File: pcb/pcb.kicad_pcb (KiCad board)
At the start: 2 copper layers, 32 x 39 mm, 88 parts, among them U1 JM20330, U2 SM2258XT, U3 FlashBGA152, U4 Conn_41PIN, U5 SY8008, U6 SY8008, U7 TX4314, Y1 25MHz, Y2 50MHz

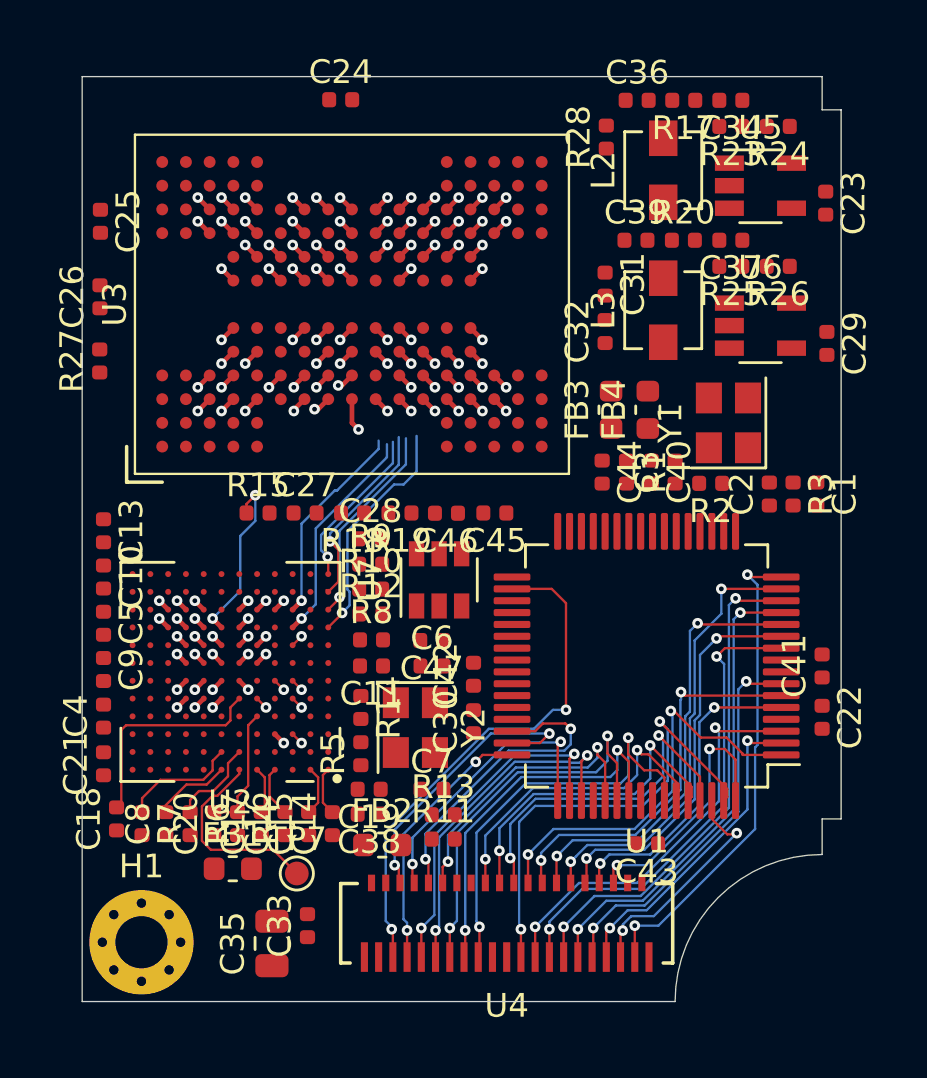
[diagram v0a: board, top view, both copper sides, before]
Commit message: Working on layout
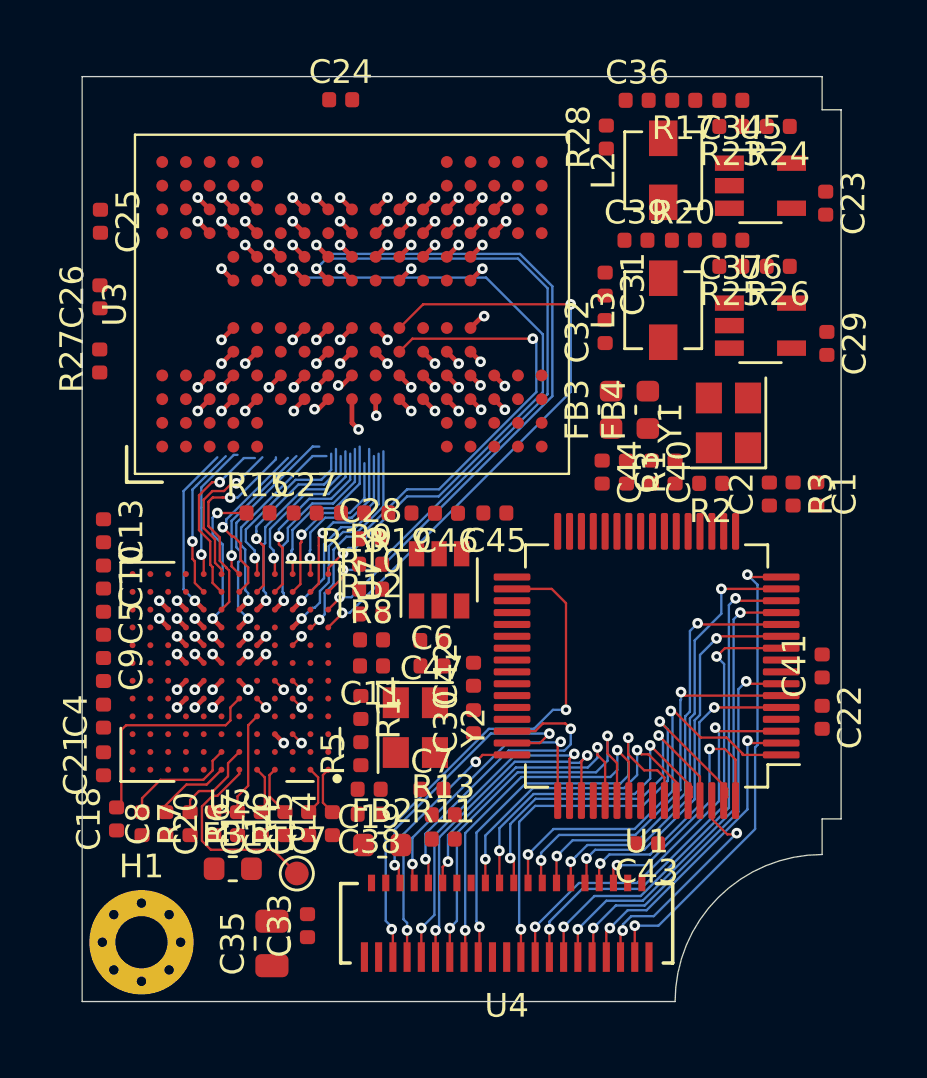
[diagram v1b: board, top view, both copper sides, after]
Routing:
- net /F0CE1: track 0.71 -> 23.3 mm, vias 1 -> 2
- net /F1CE0: track 9.29 -> 29.2 mm
- net /F1CE2: track 8.86 -> 28.6 mm
- net /F1CE3: track 7.66 -> 27.2 mm
- net /F0CE3: track 10.6 -> 25.7 mm
- net Net-(U2-PadJ6): track 1.94 -> 11.1 mm
- net /F0CLE: track 0.71 -> 9.42 mm, vias 1 -> 2
- net /F0D7: track 0.71 -> 9.00 mm, vias 1 -> 2
- net /F0D4: track 1.24 -> 9.33 mm
- net /F0ALE: track 1.24 -> 9.29 mm
- net /F0D6: track 1.24 -> 9.29 mm
- net /F0D5: track 0.71 -> 8.52 mm, vias 1 -> 2
- net /F1D7: track 0.00 -> 7.47 mm, vias 0 -> 1
- net /F0WEN: track 0.00 -> 7.43 mm, vias 0 -> 1
- net /F0DQS: track 0.00 -> 7.40 mm, vias 0 -> 1
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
